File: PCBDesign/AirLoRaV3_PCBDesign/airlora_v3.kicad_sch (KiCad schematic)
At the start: 0 parts

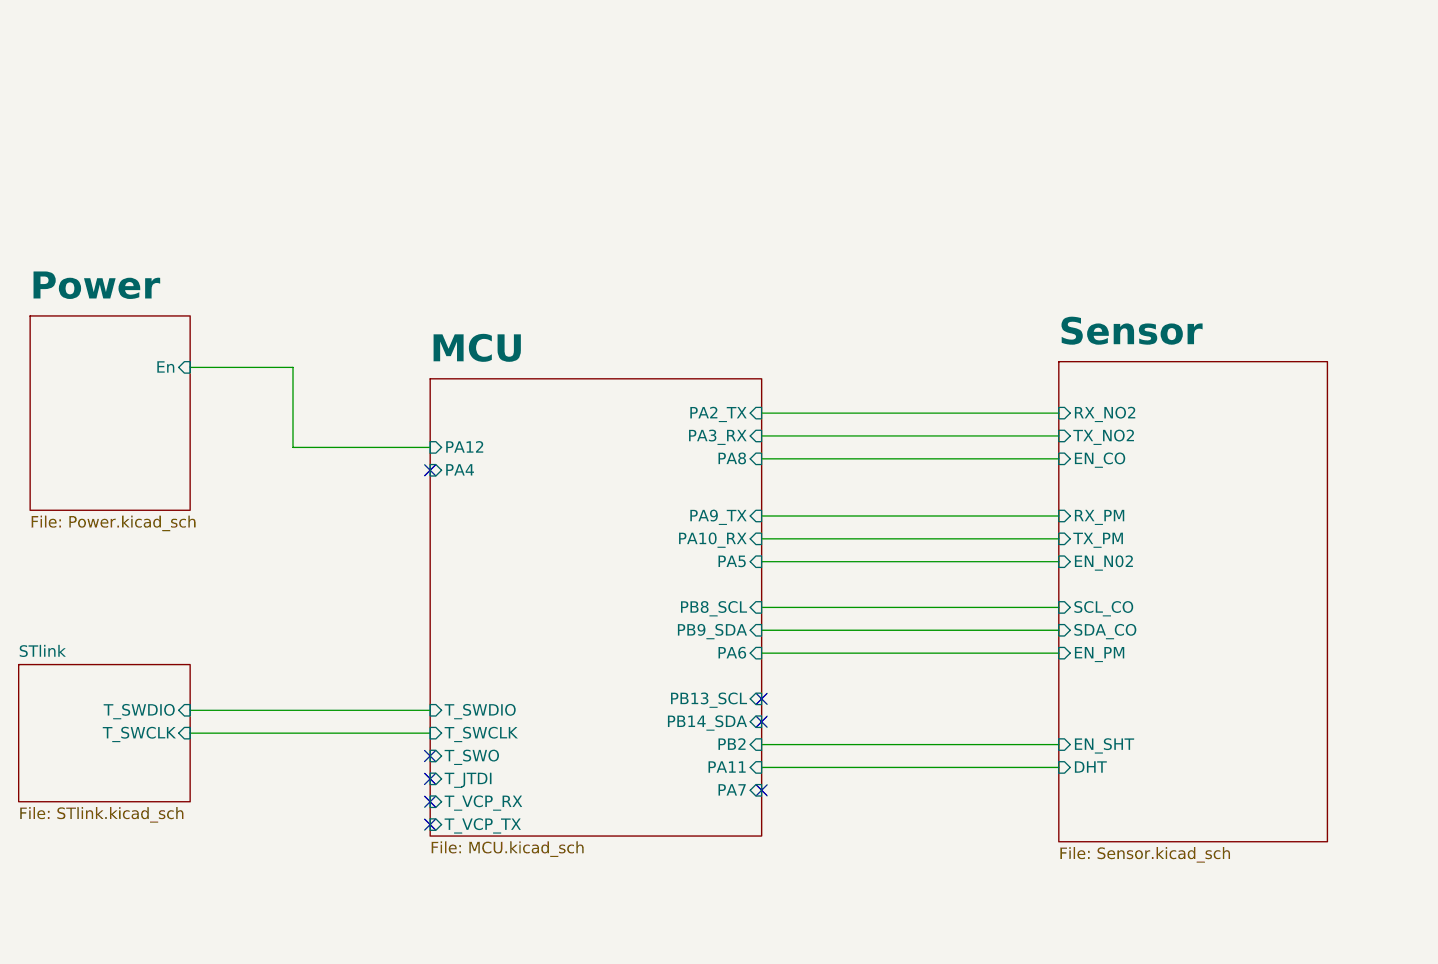
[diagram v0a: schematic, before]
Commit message: Update schematic
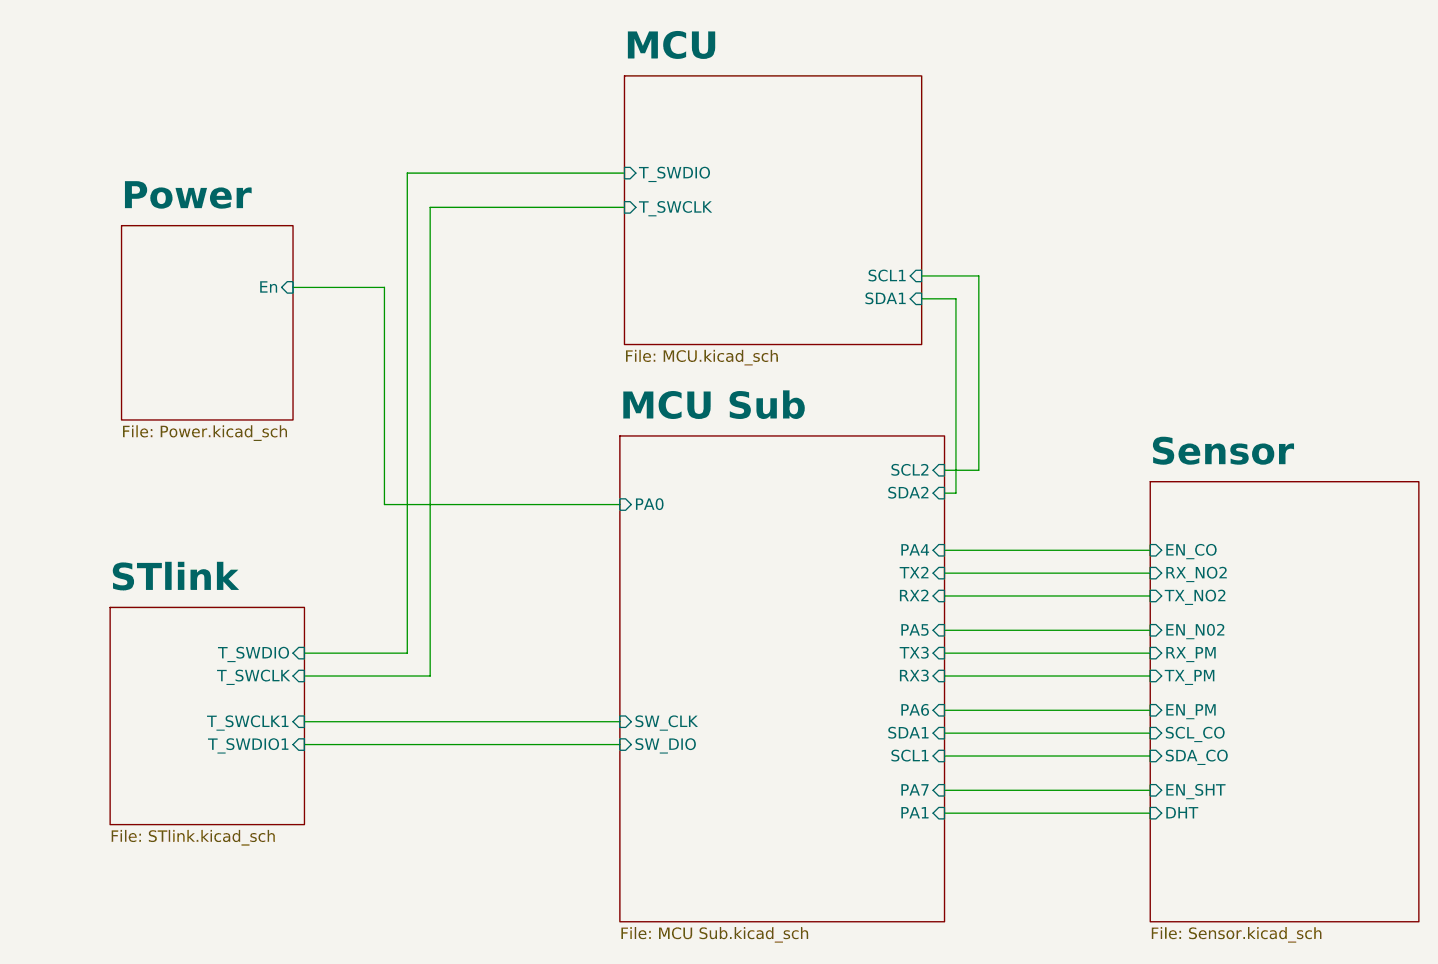
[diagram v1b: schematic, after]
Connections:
- no-connect marks 8 -> 0
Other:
- added sheet MCU Sub (MCU Sub.kicad_sch)
- sheet MCU ports: added SCL1, SDA1; removed PA10_RX, PA11, PA12, PA2_TX, PA3_RX, PA4, PA5, PA6, PA7, PA8, PA9_TX, PB13_SCL, PB14_SDA, PB2, PB8_SCL, PB9_SDA, T_JTDI, T_SWO, T_VCP_RX, T_VCP_TX
- sheet STlink ports: added T_SWCLK1, T_SWDIO1; removed none
